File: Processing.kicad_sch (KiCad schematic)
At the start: 55 parts

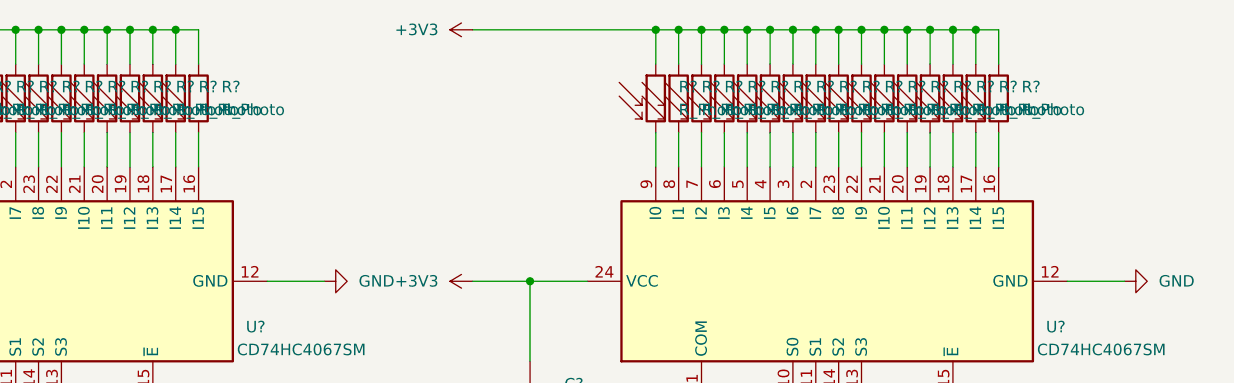
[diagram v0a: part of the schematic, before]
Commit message: 5050 - ❌ Enc - ❌ CS
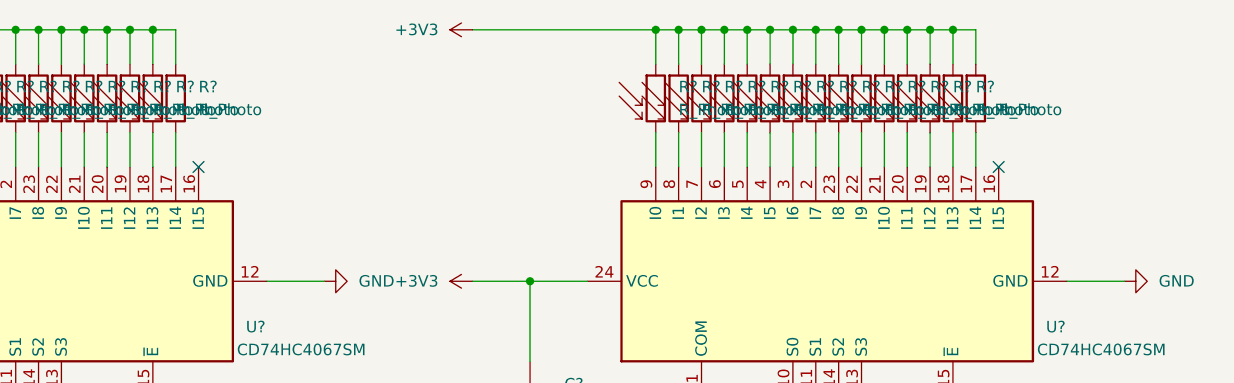
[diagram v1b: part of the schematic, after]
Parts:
- removed R? (x2): R_Photo, symbol Device:R_Photo
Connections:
- no-connect marks 21 -> 23
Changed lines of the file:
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@@
   (junction (at 60.96 24.13) (diameter 0) (color 0 0 0 0)
   )
-  (junction (at 170.18 24.13) (diameter 0) (color 0 0 0 0)
-  )
   (junction (at 95.25 173.99) (diameter 0) (color 0 0 0 0)
   )
@@
   (junction (at 31.75 52.07) (diameter 0) (color 0 0 0 0)
   )
-  (junction (at 81.28 24.13) (diameter 0) (color 0 0 0 0)
-  )
   (junction (at 85.09 186.69) (diameter 0) (color 0 0 0 0)
   )
@@
   )
   (no_connect (at 111.76 165.1))
+  (no_connect (at 83.82 39.37))
   (no_connect (at 144.78 132.08))
   (no_connect (at 111.76 160.02))
+  (no_connect (at 172.72 39.37))
   (no_connect (at 111.76 152.4))
   (no_connect (at 144.78 124.46))
@@
     (stroke (width 0) (type default))
   )
-  (wire (pts (xy 172.72 24.13) (xy 170.18 24.13))
-    (stroke (width 0) (type default))
-  )
   (wire (pts (xy 78.74 35.56) (xy 78.74 39.37))
     (stroke (width 0) (type default))
@@
     (stroke (width 0) (type default))
   )
-  (wire (pts (xy 172.72 35.56) (xy 172.72 39.37))
-    (stroke (width 0) (type default))
-  )
   (wire (pts (xy 91.44 52.07) (xy 97.79 52.07))
     (stroke (width 0) (type default))
@@
     (stroke (width 0) (type default))
   )
-  (wire (pts (xy 83.82 35.56) (xy 83.82 39.37))
-    (stroke (width 0) (type default))
-  )
   (wire (pts (xy 144.78 35.56) (xy 144.78 39.37))
     (stroke (width 0) (type default))
@@
     (stroke (width 0) (type default))
   )
-  (wire (pts (xy 172.72 24.13) (xy 172.72 27.94))
-    (stroke (width 0) (type default))
-  )
   (wire (pts (xy 81.28 24.13) (xy 78.74 24.13))
     (stroke (width 0) (type default))
@@
     (stroke (width 0) (type default))
   )
-  (wire (pts (xy 83.82 24.13) (xy 81.28 24.13))
-    (stroke (width 0) (type default))
-  )
   (wire (pts (xy 144.78 24.13) (xy 144.78 27.94))
     (stroke (width 0) (type default))
@@
   )
   (wire (pts (xy 120.65 52.07) (xy 127 52.07))
-    (stroke (width 0) (type default))
-  )
-  (wire (pts (xy 83.82 24.13) (xy 83.82 27.94))
     (stroke (width 0) (type default))
   )
@@
     )
   )
-  (symbol (lib_id "Device:R_Photo") (at 83.82 31.75 0) (unit 1)
-    (in_bom yes) (on_board yes) (dnp no) (fields_autoplaced)
-    (property "Reference" "R?" (at 86.36 30.4799 0)
-      (effects (font (size 1.27 1.27)) (justify left))
-    )
-    (property "Value" "R_Photo" (at 86.36 33.0199 0)
-      (effects (font (size 1.27 1.27)) (justify left))
-    )
-    (property "Footprint" "" (at 85.09 38.1 90)
-      (effects (font (size 1.27 1.27)) (justify left) hide)
-    )
-    (property "Datasheet" "~" (at 83.82 33.02 0)
-      (effects (font (size 1.27 1.27)) hide)
-    )
-    (pin "1")
-    (pin "2")
-    (instances
-      (project "2024l1"
-        (path "/5be543b5-1bdc-438f-a916-f916127c0a2b"
-          (reference "R?") (unit 1)
-        )
-        (path "/5be543b5-1bdc-438f-a916-f916127c0a2b/b3daf402-5eb6-40d4-a766-b970792273e4"
-          (reference "R?") (unit 1)
-        )
-      )
-    )
-  )
   (symbol (lib_id "Device:R_Photo") (at 58.42 31.75 0) (unit 1)
     (in_bom yes) (on_board yes) (dnp no) (fields_autoplaced)
@@
     (in_bom yes) (on_board yes) (dnp no) (fields_autoplaced)
     (property "Reference" "R?" (at 172.72 30.4799 0)
-      (effects (font (size 1.27 1.27)) (justify left))
+      (effects (font (size 1.27 1.27)) (justify left) hide)
     )
     (property "Value" "R_Photo" (at 172.72 33.0199 0)
@@
         )
       )
-    )
-  )
-  (symbol (lib_id "Device:R_Photo") (at 172.72 31.75 0) (unit 1)
-    (in_bom yes) (on_board yes) (dnp no) (fields_autoplaced)
-    (property "Reference" "R?" (at 175.26 30.4799 0)
-      (effects (font (size 1.27 1.27)) (justify left))
-    )
-    (property "Value" "R_Photo" (at 175.26 33.0199 0)
-      (effects (font (size 1.27 1.27)) (justify left))
-    )
-    (property "Footprint" "" (at 173.99 38.1 90)
-      (effects (font (size 1.27 1.27)) (justify left) hide)
-    )
-    (property "Datasheet" "~" (at 172.72 33.02 0)
-      (effects (font (size 1.27 1.27)) hide)
-    )
-    (pin "1")
-    (pin "2")
-    (instances
-      (project "2024l1"
-        (path "/5be543b5-1bdc-438f-a916-f916127c0a2b"
-          (reference "R?") (unit 1)
-        )
-        (path "/5be543b5-1bdc-438f-a916-f916127c0a2b/b3daf402-5eb6-40d4-a766-b970792273e4"
-          (reference "R?") (unit 1)
-        )
-      )
